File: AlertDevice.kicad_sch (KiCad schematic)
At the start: 9 parts, among them Q38 2N2222, Q39 2N2222

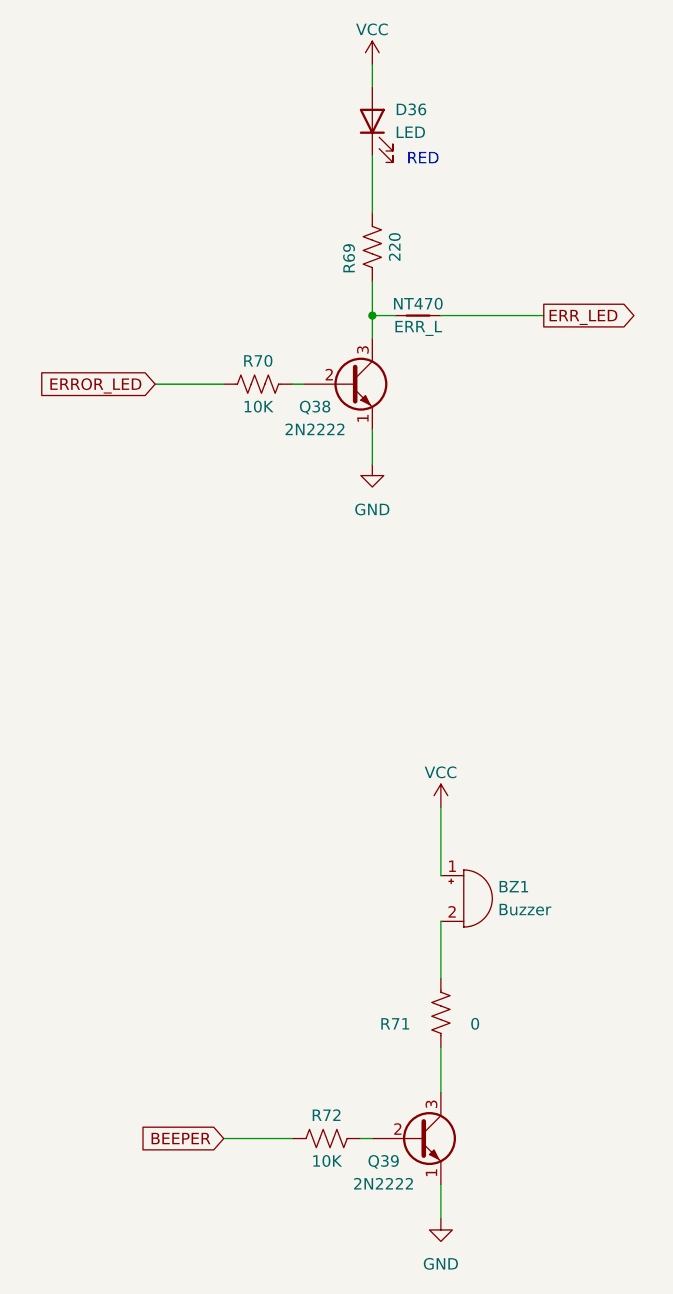
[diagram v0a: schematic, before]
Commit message: backup 1 bank done
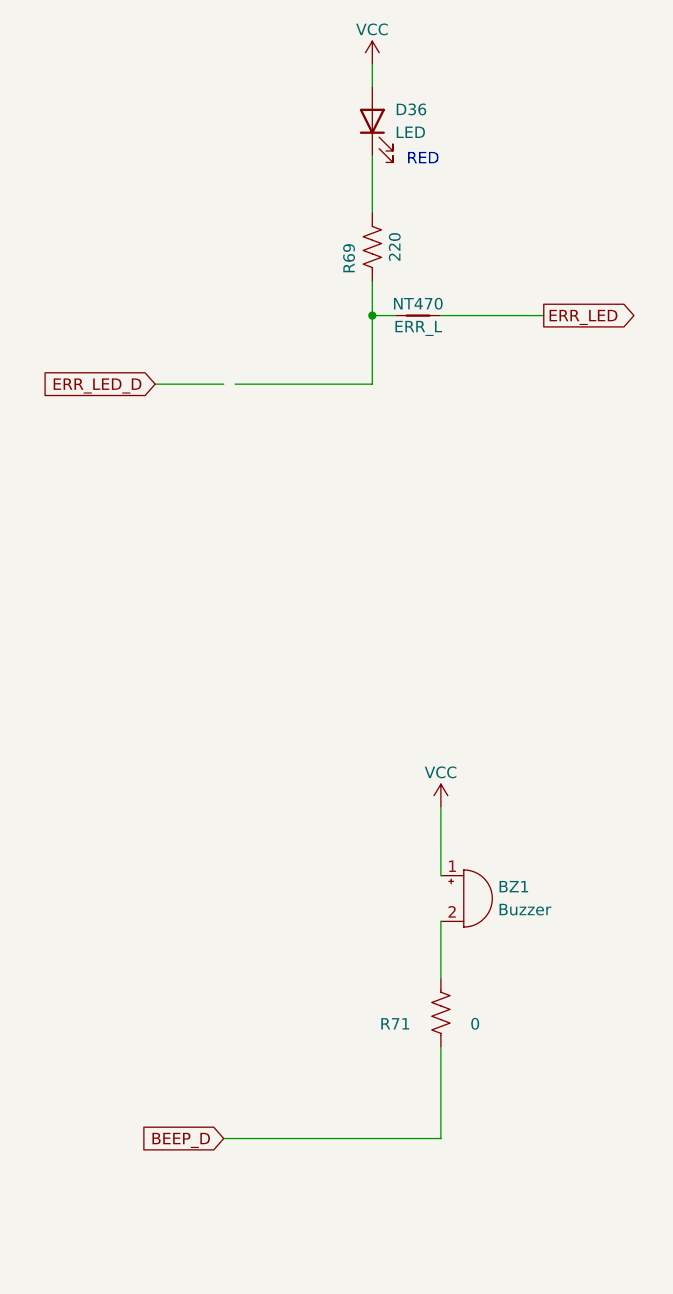
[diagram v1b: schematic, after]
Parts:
- removed Q38, Q39: 2N2222, Package_TO_SOT_THT:TO-92_Inline, symbol Transistor_BJT:2N3904
- removed R70, R72: 10K, Resistor_THT:R_Axial_DIN0309_L9.0mm_D3.2mm_P12.70mm_Horizontal, symbol Device:R_US
- NT470: footprint NetTie:NetTie-2_THT_Pad1.0mm -> NetTie:NetTie-2_Front1.0mm
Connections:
- net BEEP_D: now reaches R71.1
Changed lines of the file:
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@@
+    (stroke (width 0) (type default) (color 0 0 0 0))
+  )
+  (wire (pts (xy 68.58 64.77) (xy 83.82 64.77))
     (stroke (width 0) (type default) (color 0 0 0 0))
   )
@@
     (stroke (width 0) (type default) (color 0 0 0 0))
   )
-  (wire (pts (xy 91.44 138.43) (xy 91.44 143.51))
-    (stroke (width 0) (type default) (color 0 0 0 0))
-  )
-  (wire (pts (xy 82.55 148.59) (xy 83.82 148.59))
-    (stroke (width 0) (type default) (color 0 0 0 0))
-  )
-  (wire (pts (xy 91.44 153.67) (xy 91.44 157.48))
-    (stroke (width 0) (type default) (color 0 0 0 0))
-  )
   (wire (pts (xy 91.44 57.15) (xy 102.87 57.15))
     (stroke (width 0) (type default) (color 0 0 0 0))
   )
+  (wire (pts (xy 91.44 138.43) (xy 91.44 148.59))
+    (stroke (width 0) (type default) (color 0 0 0 0))
+  )
   (wire (pts (xy 83.82 29.21) (xy 83.82 31.75))
     (stroke (width 0) (type default) (color 0 0 0 0))
   )
-  (wire (pts (xy 67.31 148.59) (xy 74.93 148.59))
-    (stroke (width 0) (type default) (color 0 0 0 0))
-  )
-  (wire (pts (xy 74.93 64.77) (xy 76.2 64.77))
+  (wire (pts (xy 67.31 148.59) (xy 91.44 148.59))
     (stroke (width 0) (type default) (color 0 0 0 0))
   )
@@
     (stroke (width 0) (type default) (color 0 0 0 0))
   )
-  (wire (pts (xy 83.82 69.85) (xy 83.82 73.66))
-    (stroke (width 0) (type default) (color 0 0 0 0))
-  )
-  (wire (pts (xy 83.82 57.15) (xy 83.82 59.69))
+  (wire (pts (xy 83.82 57.15) (xy 83.82 64.77))
     (stroke (width 0) (type default) (color 0 0 0 0))
   )
@@
     (effects (font (size 1.27 1.27)) (justify left bottom))
   )
-  (global_label "BEEPER" (shape input) (at 67.31 148.59 180) (fields_autoplaced)
+  (global_label "BEEP_D" (shape input) (at 67.31 148.59 180) (fields_autoplaced)
     (effects (font (size 1.27 1.27)) (justify right))
-    (property "Intersheet References" "${INTERSHEET_REFS}" (id 0) (at 57.6398 148.5106 0)
+    (property "Intersheet References" "${INTERSHEET_REFS}" (id 0) (at 57.8212 148.5106 0)
       (effects (font (size 1.27 1.27)) (justify right) hide)
     )
   )
-  (global_label "ERROR_LED" (shape input) (at 59.69 64.77 180) (fields_autoplaced)
+  (global_label "ERR_LED_D" (shape input) (at 59.69 64.77 180) (fields_autoplaced)
     (effects (font (size 1.27 1.27)) (justify right))
-    (property "Intersheet References" "${INTERSHEET_REFS}" (id 0) (at 46.5726 64.6906 0)
+    (property "Intersheet References" "${INTERSHEET_REFS}" (id 0) (at 46.9355 64.6906 0)
       (effects (font (size 1.27 1.27)) (justify right) hide)
     )
@@
       (effects (font (size 1.27 1.27)) (justify left) hide)
     )
-  )
-  (symbol (lib_id "power:GND") (at 91.44 157.48 0) (unit 1)
-    (in_bom yes) (on_board yes) (fields_autoplaced)
-    (property "Reference" "#PWR0122" (id 0) (at 91.44 163.83 0)
-      (effects (font (size 1.27 1.27)) hide)
-    )
-    (property "Value" "GND" (id 1) (at 91.44 162.56 0))
-    (property "Footprint" "" (id 2) (at 91.44 157.48 0)
-      (effects (font (size 1.27 1.27)) hide)
-    )
-    (property "Datasheet" "" (id 3) (at 91.44 157.48 0)
-      (effects (font (size 1.27 1.27)) hide)
-    )
-    (pin "1")
-  )
-  (symbol (lib_id "Device:R_US") (at 78.74 148.59 270) (unit 1)
-    (in_bom yes) (on_board yes)
-    (property "Reference" "R72" (id 0) (at 78.74 146.05 90))
-    (property "Value" "10K" (id 1) (at 78.74 151.13 90))
-    (property "Footprint" "Resistor_THT:R_Axial_DIN0309_L9.0mm_D3.2mm_P12.70mm_Horizontal" (id 2) (at 78.486 149.606 90)
-      (effects (font (size 1.27 1.27)) hide)
-    )
-    (property "Datasheet" "~" (id 3) (at 78.74 148.59 0)
-      (effects (font (size 1.27 1.27)) hide)
-    )
-    (pin "1")
-    (pin "2")
   )
   (symbol (lib_id "Device:R_US") (at 83.82 49.53 180) (unit 1)
@@
     (pin "1")
   )
-  (symbol (lib_id "Device:R_US") (at 71.12 64.77 270) (unit 1)
-    (in_bom yes) (on_board yes)
-    (property "Reference" "R70" (id 0) (at 71.12 62.23 90))
-    (property "Value" "10K" (id 1) (at 71.12 67.31 90))
-    (property "Footprint" "Resistor_THT:R_Axial_DIN0309_L9.0mm_D3.2mm_P12.70mm_Horizontal" (id 2) (at 70.866 65.786 90)
-      (effects (font (size 1.27 1.27)) hide)
-    )
-    (property "Datasheet" "~" (id 3) (at 71.12 64.77 0)
-      (effects (font (size 1.27 1.27)) hide)
-    )
-    (pin "1")
-    (pin "2")
-  )
   (symbol (lib_id "Device:LED") (at 83.82 35.56 90) (unit 1)
     (in_bom yes) (on_board yes)
@@
     (pin "2")
   )
-  (symbol (lib_id "power:GND") (at 83.82 73.66 0) (unit 1)
-    (in_bom yes) (on_board yes) (fields_autoplaced)
-    (property "Reference" "#PWR0120" (id 0) (at 83.82 80.01 0)
-      (effects (font (size 1.27 1.27)) hide)
-    )
-    (property "Value" "GND" (id 1) (at 83.82 78.74 0))
-    (property "Footprint" "" (id 2) (at 83.82 73.66 0)
-      (effects (font (size 1.27 1.27)) hide)
-    )
-    (property "Datasheet" "" (id 3) (at 83.82 73.66 0)
-      (effects (font (size 1.27 1.27)) hide)
-    )
-    (pin "1")
-  )
   (symbol (lib_id "Device:NetTie_2") (at 88.9 57.15 0) (unit 1)
     (in_bom yes) (on_board yes)
     (property "Reference" "NT470" (id 0) (at 88.9 55.88 0))
     (property "Value" "ERR_L" (id 1) (at 88.9 58.42 0))
-    (property "Footprint" "NetTie:NetTie-2_THT_Pad1.0mm" (id 2) (at 88.9 57.15 0)
+    (property "Footprint" "NetTie:NetTie-2_Front1.0mm" (id 2) (at 88.9 57.15 0)
       (effects (font (size 1.27 1.27)) hide)
     )
@@
     (pin "2")
   )
-  (symbol (lib_id "Transistor_BJT:2N3904") (at 88.9 148.59 0) (unit 1)
-    (in_bom yes) (on_board yes)
-    (property "Reference" "Q39" (id 0) (at 85.09 151.13 0))
-    (property "Value" "2N2222" (id 1) (at 85.09 153.67 0))
-    (property "Footprint" "Package_TO_SOT_THT:TO-92_Inline" (id 2) (at 93.98 150.495 0)
-      (effects (font (size 1.27 1.27) italic) (justify left) hide)
-    )
-    (property "Datasheet" "https://www.onsemi.com/pub/Collateral/2N3903-D.PDF" (id 3) (at 88.9 148.59 0)
-      (effects (font (size 1.27 1.27)) (justify left) hide)
-    )
-    (pin "1")
-    (pin "2")
-    (pin "3")
-  )
-  (symbol (lib_id "Transistor_BJT:2N3904") (at 81.28 64.77 0) (unit 1)
-    (in_bom yes) (on_board yes)
-    (property "Reference" "Q38" (id 0) (at 77.47 67.31 0))
-    (property "Value" "2N2222" (id 1) (at 77.47 69.85 0))
-    (property "Footprint" "Package_TO_SOT_THT:TO-92_Inline" (id 2) (at 86.36 66.675 0)
-      (effects (font (size 1.27 1.27) italic) (justify left) hide)
-    )
-    (property "Datasheet" "https://www.onsemi.com/pub/Collateral/2N3903-D.PDF" (id 3) (at 81.28 64.77 0)
-      (effects (font (size 1.27 1.27)) (justify left) hide)
-    )
-    (pin "1")
-    (pin "2")
-    (pin "3")
-  )
   (symbol (lib_id "power:VCC") (at 91.44 111.76 0) (unit 1)
